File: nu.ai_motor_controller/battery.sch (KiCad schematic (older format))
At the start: 44 parts, among them J12 XT60_RA_MALE, J13 S4B-XH-A, J14 NP_Screw_Terminal_01x02, J15 XT60_RA_MALE, J16 S4B-XH-A, J17 S4B-XH-A, J18 XT60_RA_FEMALE, Q1 IRF9540N, Q2 SSM3K35AMFV, Q4 SSM3K35AMFV, Q5 SSM3K35AMFV, Q6 SSM3K35AMFV, SW2 TACTILE_SWITCH, SW3 TACTILE_SWITCH

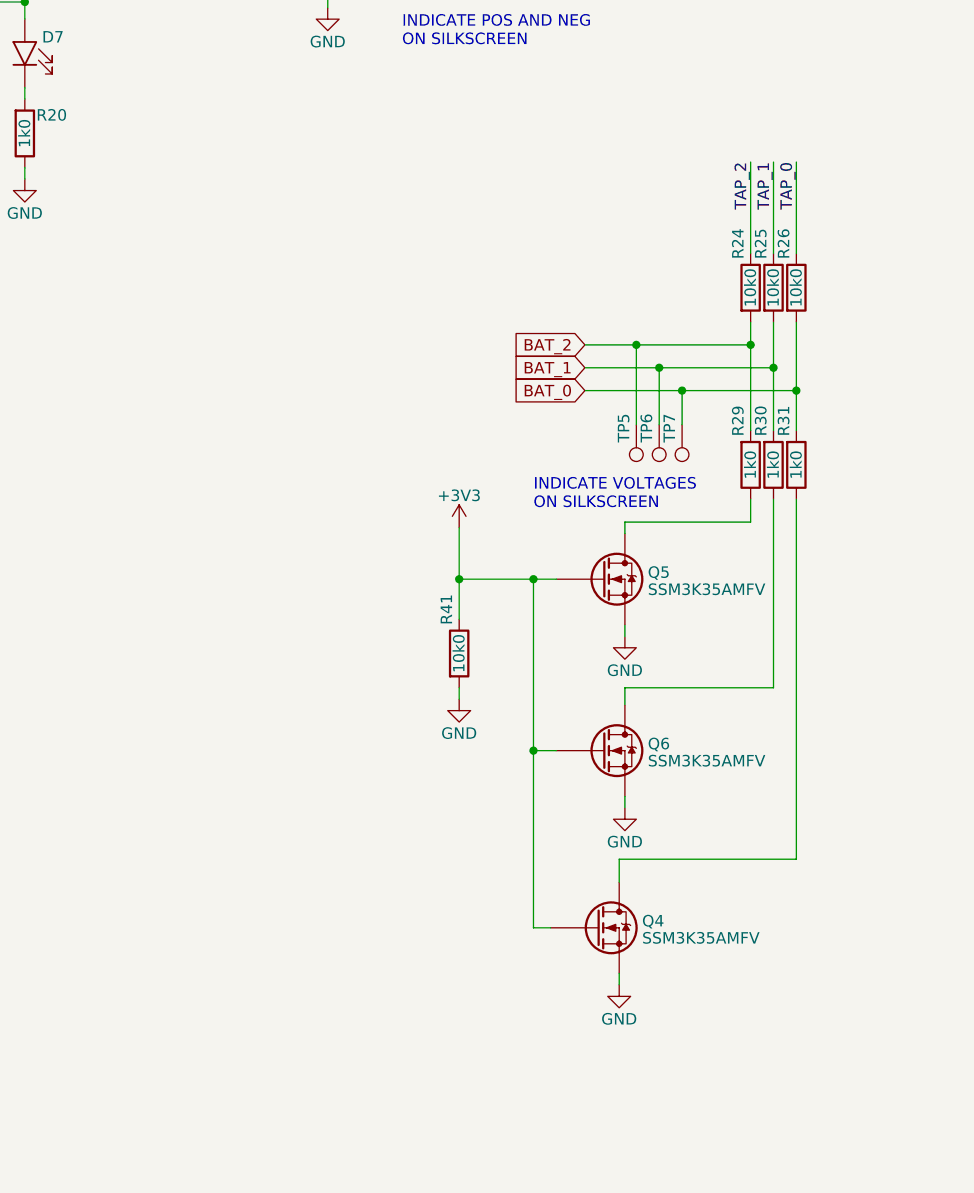
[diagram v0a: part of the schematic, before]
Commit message: automated commit
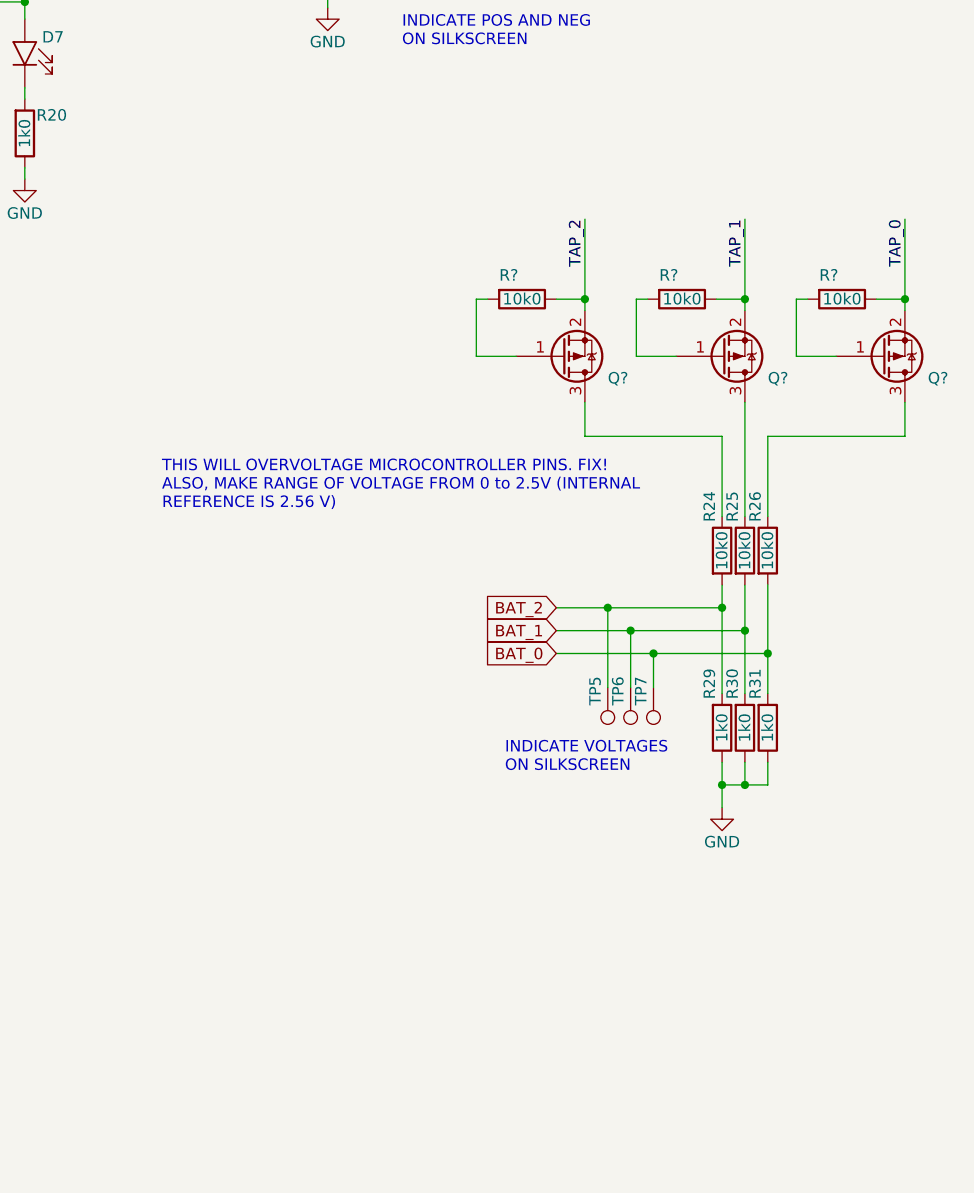
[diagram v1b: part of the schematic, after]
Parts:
- removed Q4, Q5, Q6: SSM3K35AMFV, Package_TO_SOT_SMD:SOT-723, symbol custom:SSM3K35AMFV
- removed R41: CR0603-JW-103ELF, Resistor_SMD:R_0603_1608Metric, symbol custom:CR0603-JW-103ELF
- added Q? (x3): AO3407A, Package_TO_SOT_SMD:SOT-23, symbol custom:AO3407A
- added R? (x3): CR0603-JW-103ELF, Resistor_SMD:R_0603_1608Metric, symbol custom:CR0603-JW-103ELF
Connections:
- net GND: now also R29.2, R30.2, R31.2
- net TAP_0: now also Q?.2 (S), R?.1; no longer R26.1
- net TAP_1: now also Q?.2 (S), R?.1; no longer R25.1
- net TAP_2: now also Q?.2 (S), R?.1; no longer R24.1
- new net: Q?.3 (D), R25.1
- new net: Q?.3 (D), R26.1
- new net: Q?.3 (D), R24.1
- new net: Q?.1 (G), R?.2 (x3)
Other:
- note added: "THIS WILL OVERVOLTAGE MICROCONTROLLER PINS. FIX!\nALSO, MAKE RANGE OF VOLTAGE FROM 0 to 2.5V (INTERNAL\nREFERENCE IS 2.56 V)"
- moved on the sheet: R24, R25, R26, R29, R30, R31, TP5, TP6, TP7

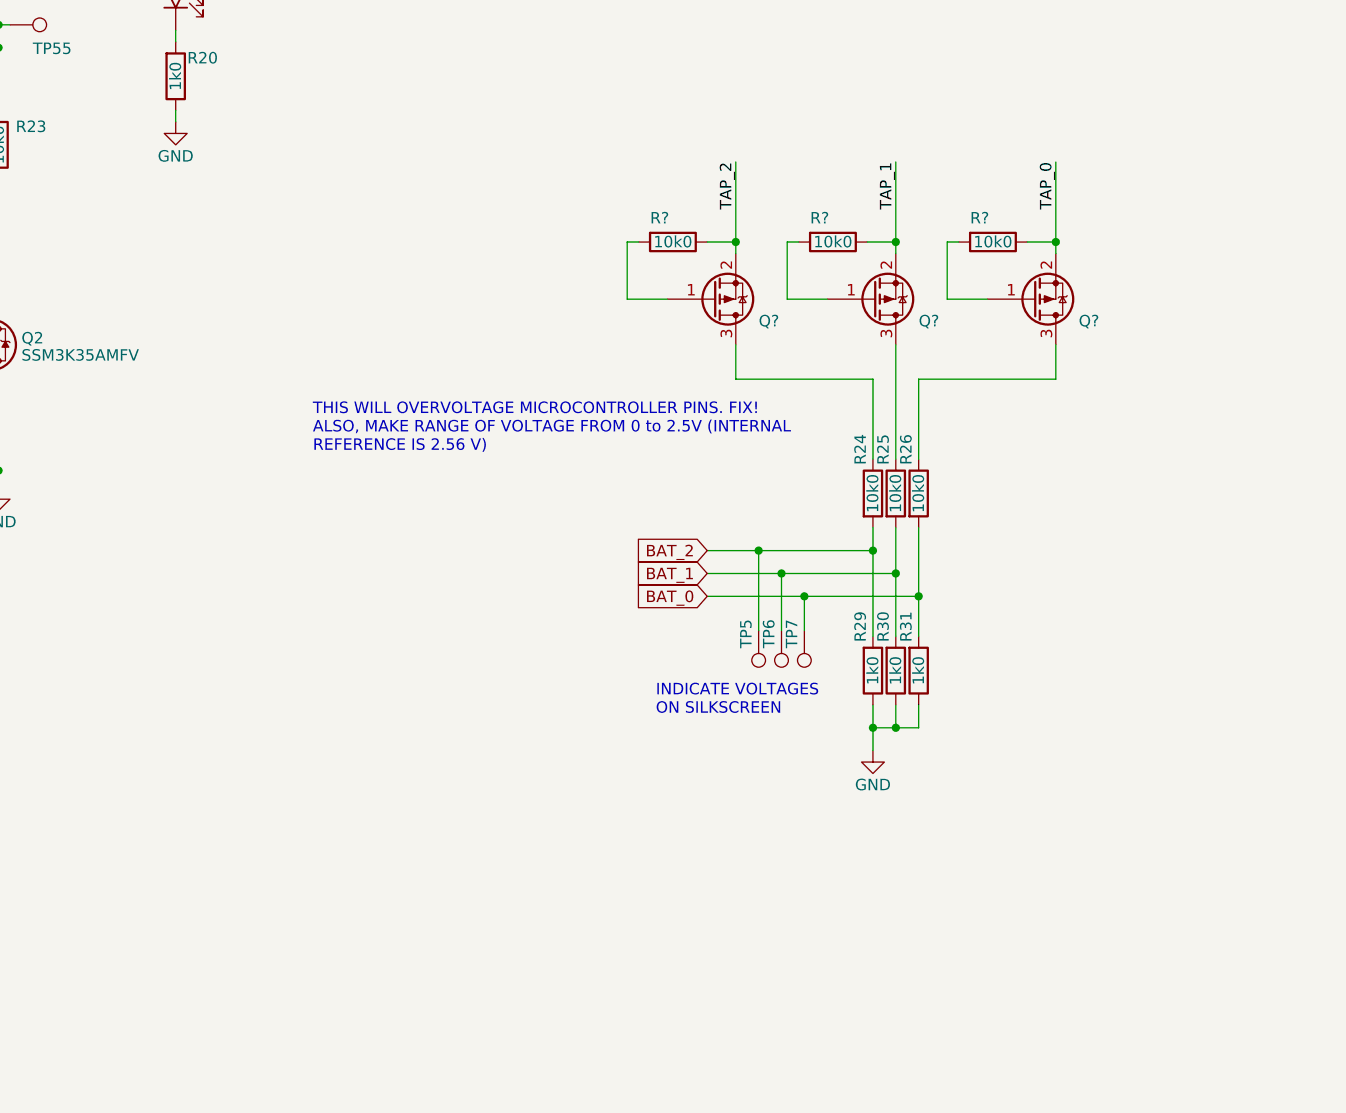
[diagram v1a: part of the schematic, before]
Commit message: automated commit
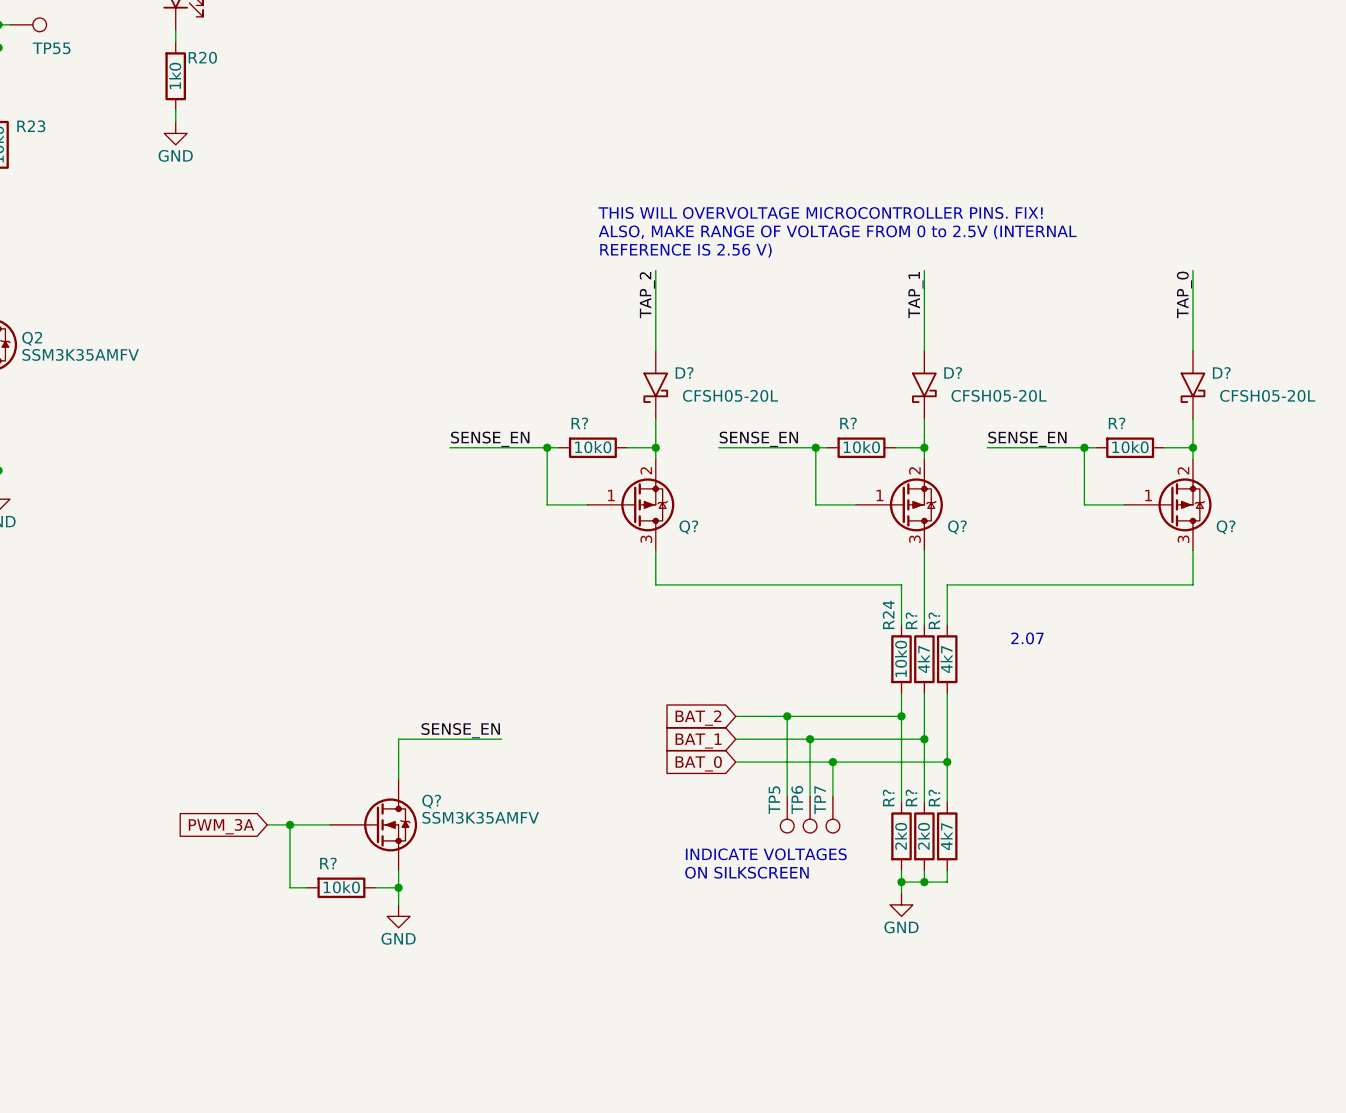
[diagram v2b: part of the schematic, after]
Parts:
- removed R25, R26: CR0603-JW-103ELF, Resistor_SMD:R_0603_1608Metric, symbol custom:CR0603-JW-103ELF
- removed R29, R30, R31: RC0603JR-071KL, Resistor_SMD:R_0603_1608Metric, symbol custom:RC0603JR-071KL
- added D? (x3): CFSH05-20L, custom:SOD-882, symbol custom:CFSH05-20L
- added Q?: SSM3K35AMFV, Package_TO_SOT_SMD:SOT-723, symbol custom:SSM3K35AMFV
- added R? (x2): RMCF0603FT2K00, Resistor_SMD:R_0603_1608Metric, symbol custom:RMCF0603FT2K00
- added R?: CR0603-JW-103ELF, Resistor_SMD:R_0603_1608Metric, symbol custom:CR0603-JW-103ELF
- added R? (x3): RMCF0603FT4K70, Resistor_SMD:R_0603_1608Metric, symbol custom:RMCF0603FT4K70
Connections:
- net BAT_0: now also R?.1, R?.2
- net BAT_1: now also R?.1, R?.2
- net BAT_2: now also R?.1
- net GND: now also Q?.2 (S), R?.1, R?.2, R?.2, R?.2
- net TAP_0: now also D?.2 (A); no longer Q?.2 (S), R?.1
- net TAP_1: now also D?.2 (A); no longer Q?.2 (S), R?.1
- net TAP_2: now also D?.2 (A); no longer Q?.2 (S), R?.1
- net at Q?.3 (D): now also R?.1 (x2)
- net SENSE_EN: now reaches Q?.1 (G), R?.2
- net SENSE_EN: now also Q?.1 (G), Q?.1 (G), R?.2, R?.2, Q?.3 (D)
- new net: D?.1 (K), Q?.2 (S), R?.1 (x3)
- new net PWM_3A: Q?.1 (G), R?.2
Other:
- note added: "2.07"
- moved on the sheet: Q?, R24, R?, TP5, TP6, TP7

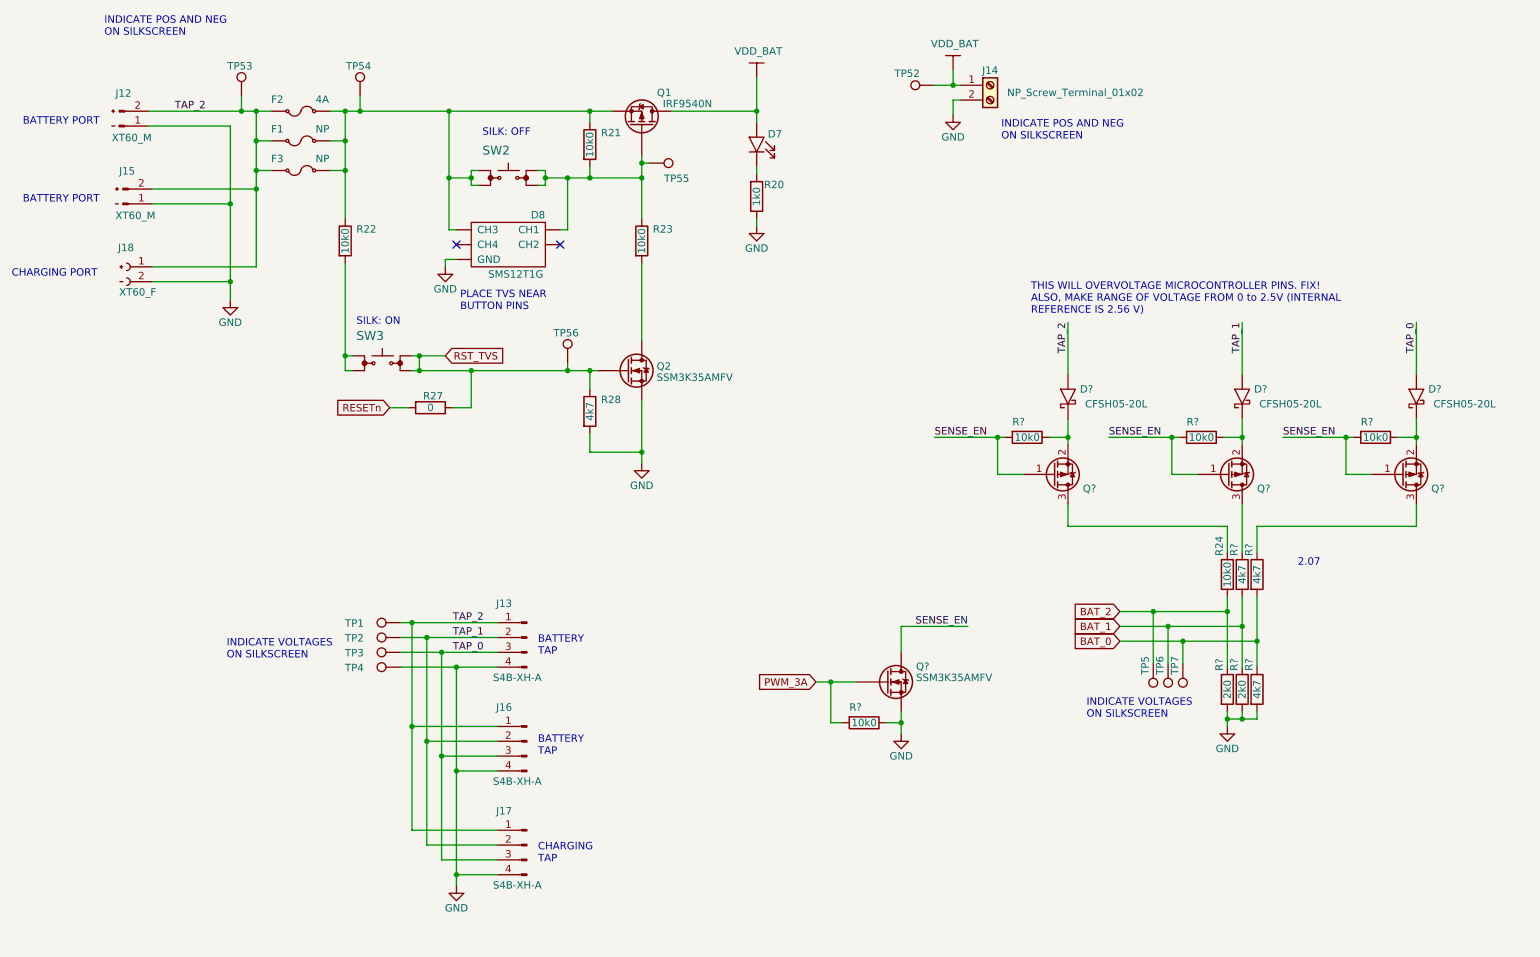
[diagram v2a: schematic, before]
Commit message: automated commit
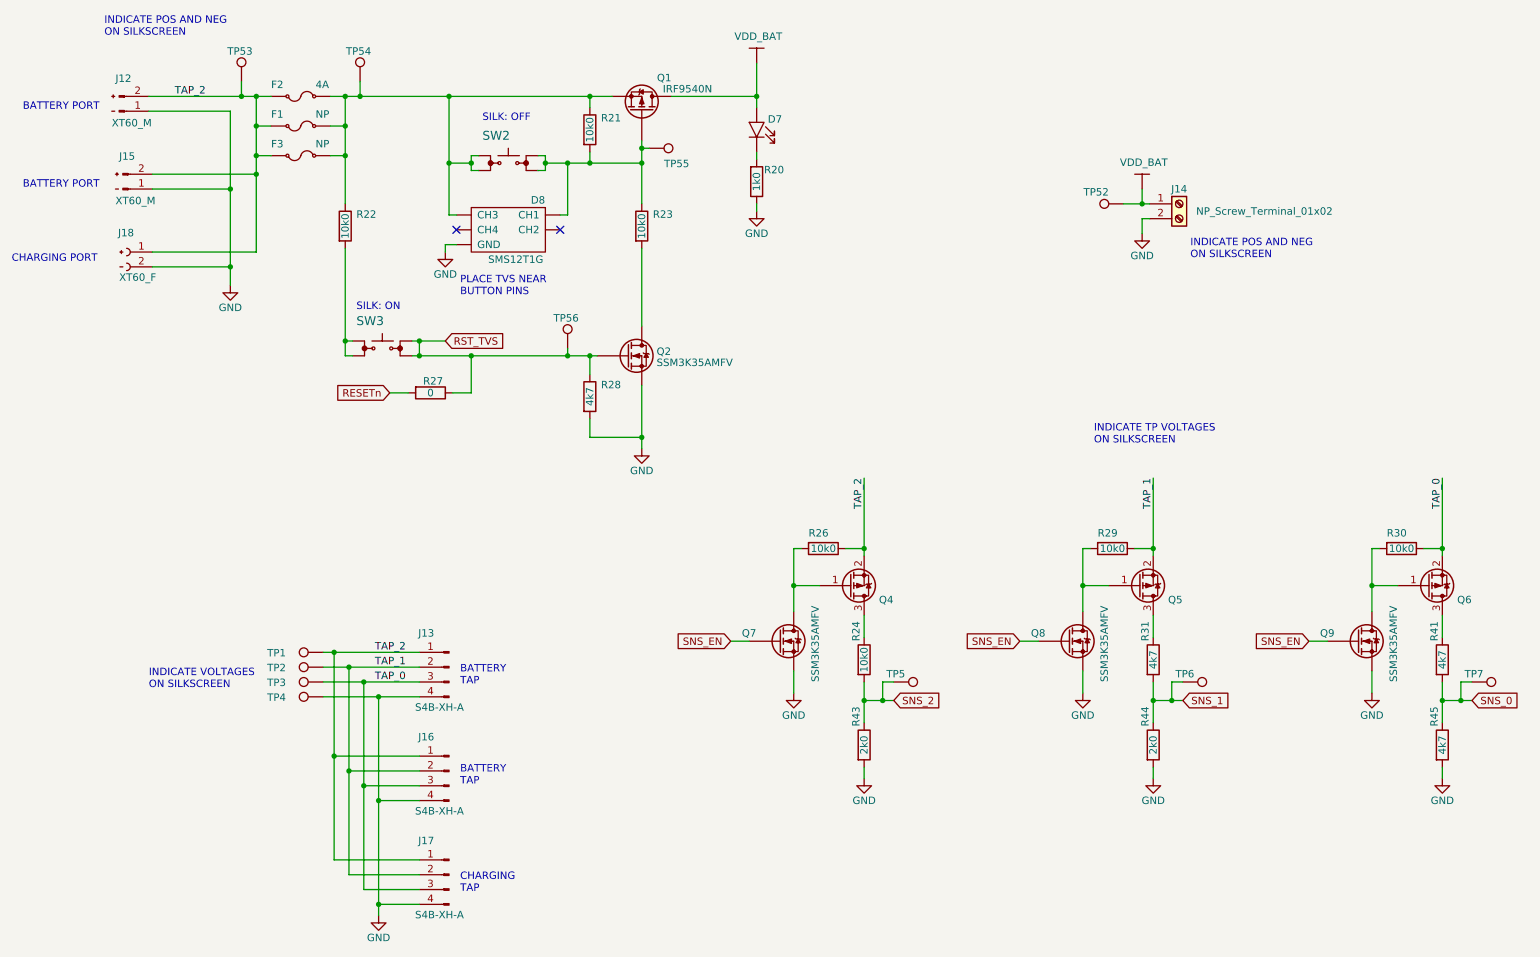
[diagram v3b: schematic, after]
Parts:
- removed D? (x3): CFSH05-20L, custom:SOD-882, symbol custom:CFSH05-20L
- removed Q? (x2): AO3407A, Package_TO_SOT_SMD:SOT-23, symbol custom:AO3407A
- removed R? (x3): CR0603-JW-103ELF, Resistor_SMD:R_0603_1608Metric, symbol custom:CR0603-JW-103ELF
- added Q5, Q6: AO3407A, Package_TO_SOT_SMD:SOT-23, symbol custom:AO3407A
- added Q8, Q9: SSM3K35AMFV, Package_TO_SOT_SMD:SOT-723, symbol custom:SSM3K35AMFV
- added R29, R30: CR0603-JW-103ELF, Resistor_SMD:R_0603_1608Metric, symbol custom:CR0603-JW-103ELF
- gave numbers to parts that had none: 8
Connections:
- net GND: now also Q8.2 (S), Q9.2 (S)
- net TAP_0: now also Q6.2 (S), R30.1
- net TAP_1: now also Q5.2 (S), R29.1
- net TAP_2: now also Q4.2 (S), R26.1
- net at R31.1: now also Q5.3 (D)
- net at R41.1: now also Q6.3 (D)
- net BAT_0 renamed SNS_0
- net BAT_1 renamed SNS_1
- net BAT_2 renamed SNS_2
- net PWM_3A renamed SNS_EN
- net SNS_EN: now also Q8.1 (G), Q9.1 (G)
- net SENSE_EN: no longer names the net of Q4.1 (G), Q7.3 (D), R26.2
- new net: Q5.1 (G), Q8.3 (D), R29.2
- new net: Q6.1 (G), Q9.3 (D), R30.2
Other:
- note added: "INDICATE TP VOLTAGES\nON SILKSCREEN"
- note removed: "2.07"
- note removed: "THIS WILL OVERVOLTAGE MICROCONTROLLER PINS. FIX!\nALSO, MAKE RANGE OF VOLTAGE FROM 0 to 2.5V (INTERNAL\nREFERENCE IS 2.56 V)"
- moved on the sheet: D7, D8, F1, F2, F3, J12, J13, J14, J15, J16, J17, J18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
